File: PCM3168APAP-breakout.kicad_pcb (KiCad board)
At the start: 4 copper layers, 133.6 x 66.2 mm, 206 parts, among them IC101 PCM3168APAP, IC102 SN74LVC2G34DRLR, J1 ~{RESET}, J101 I^{2}S, J102 I^{2}C, J103 DIN, J104 DOUT, J201 ANALOG_IN1, J202 ANALOG_IN2, J203 ANALOG_IN3, J301 OUTPUT1-4, J302 OUTPUT5-8, J401 POWER IN, U201 OPA4134UA, U202 OPA2134, U301 OPA4134UA, U302 OPA4134UA, U401 AMS1117-5.0, U402 AMS1117-3.3

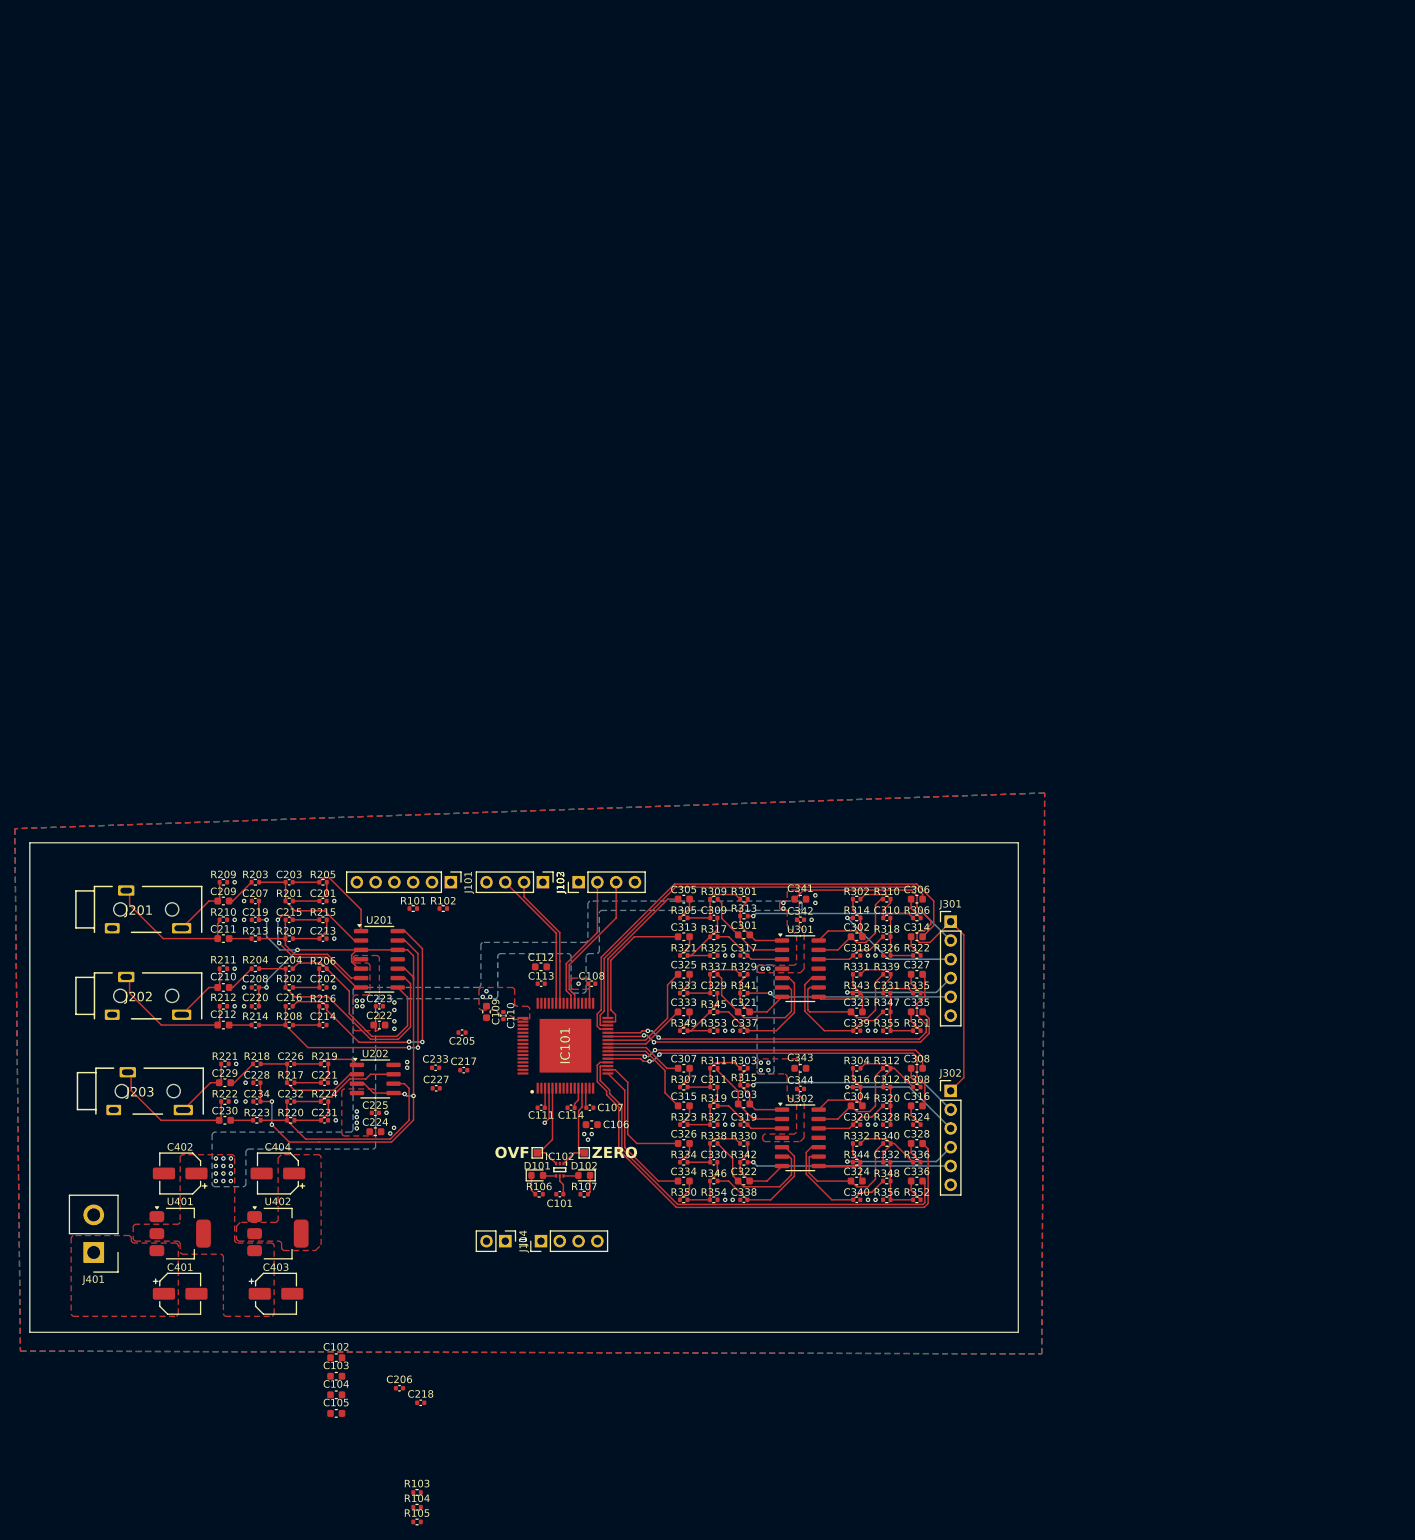
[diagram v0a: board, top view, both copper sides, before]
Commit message: finished routin, updated schematic, added PDF
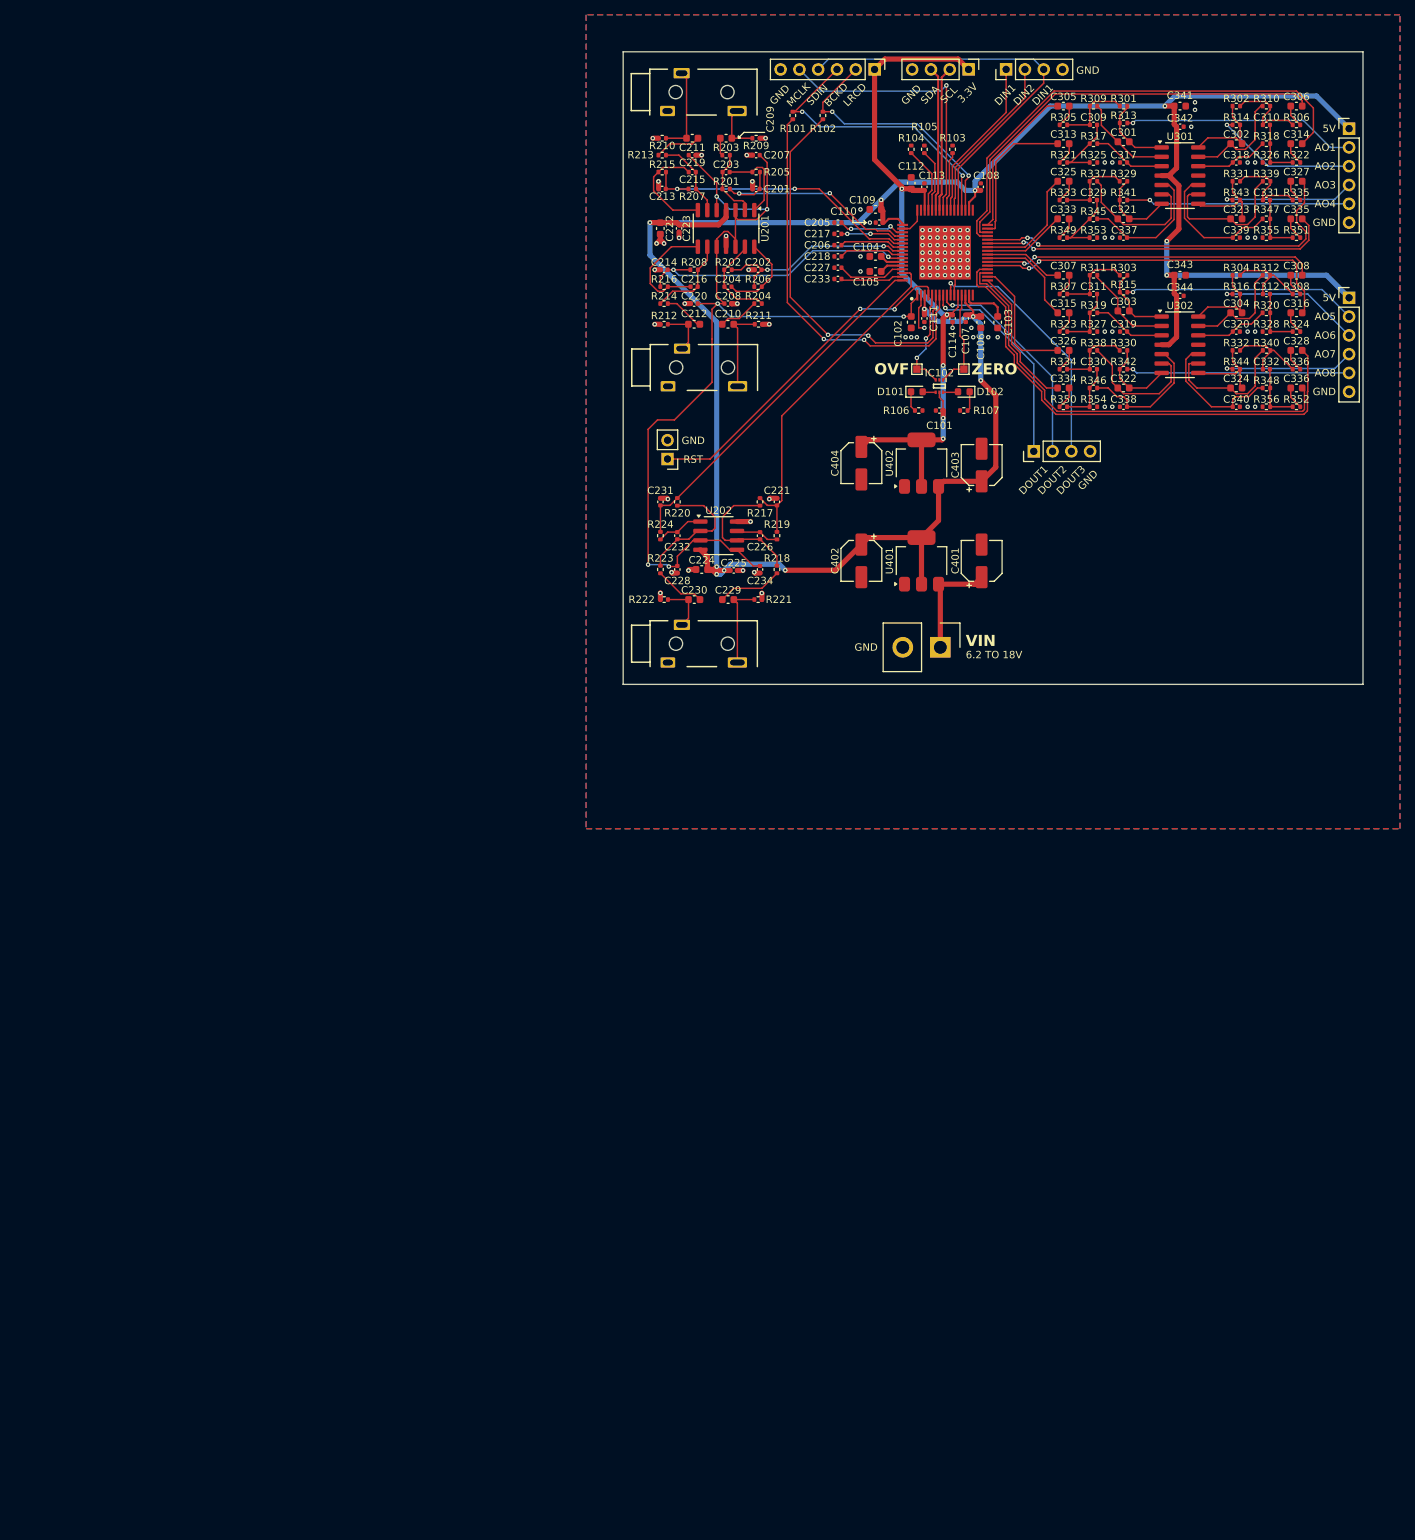
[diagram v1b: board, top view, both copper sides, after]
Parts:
- moved R105 197.8 mm to (140.7, 43.2), turned to -90 degrees
- moved R103 195.4 mm to (144.5, 43.2), turned to -90 degrees
- moved R104 195.3 mm to (138.9, 43.2), turned to -90 degrees
- moved C105 170.7 mm to (134.1, 59.7), turned to 180 degrees
- moved C104 170.3 mm to (134.1, 57.7), turned to 180 degrees
- moved C103 168.2 mm to (150.6, 66.5), turned to -90 degrees
- moved C206 165.5 mm to (129.0, 56.1), turned to 180 degrees
- moved C218 164.9 mm to (129.0, 57.7), turned to 180 degrees
- moved C102 160.1 mm to (138.9, 66.5), turned to -90 degrees
- moved C403 147.1 mm to (148.5, 85.9), turned to 90 degrees
- moved C401 146.8 mm to (148.5, 98.8), turned to 90 degrees
- moved J401 140.7 mm to (142.9, 110.5), turned to -90 degrees
- moved U402 135.7 mm to (140.3, 85.6), turned to 90 degrees
- moved U401 135.3 mm to (140.3, 98.8), turned to 90 degrees
- moved J201 133.6 mm to (106.0, 38.0)
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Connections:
- C204 pad 1: Net-(U201C--) -> Net-(U201D--)
- C216 pad 1: Net-(U201D--) -> Net-(U201C--)
- C226 pad 1: Net-(U202A--) -> Net-(U202B--)
- C232 pad 1: Net-(U202B--) -> Net-(U202A--)
- R202 pad 1: Net-(U201C--) -> Net-(U201D--)
- R204 pad 2: Net-(U201C--) -> Net-(U201D--)
- R208 pad 1: Net-(U201D--) -> Net-(U201C--)
- R214 pad 2: Net-(U201D--) -> Net-(U201C--)
- R217 pad 1: Net-(U202A--) -> Net-(U202B--)
- R218 pad 2: Net-(U202A--) -> Net-(U202B--)
- R220 pad 1: Net-(U202B--) -> Net-(U202A--)
- R223 pad 2: Net-(U202B--) -> Net-(U202A--)
- U201 pad 14: Net-(C216-Pad2) -> Net-(C204-Pad2)
- U201 pad 8: Net-(C204-Pad2) -> Net-(C216-Pad2)
- U202 pad 1: Net-(C226-Pad2) -> Net-(C232-Pad2)
- U202 pad 7: Net-(C232-Pad2) -> Net-(C226-Pad2)
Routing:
- net +5V: track 63.5 -> 344.2 mm, vias 35 -> 13
- net +3.3V: track 5.52 -> 99.4 mm, vias 0 -> 5
- net /SDIN: track 0.00 -> 55.5 mm
- net /BCK_ADC: track 0.00 -> 54.1 mm, vias 0 -> 2
- net /LRCK_ADC: track 0.00 -> 53.9 mm, vias 0 -> 2
- net /Analog Inputs/VIN6+: track 6.53 -> 48.9 mm
- net /~{RST}: track 4.93 -> 46.2 mm, vias 1 -> 2
- net /Analog Inputs/VIN5+: track 6.53 -> 46.3 mm
- net /BCK_DAC: track 0.00 -> 39.6 mm, vias 0 -> 2
- net /Analog Inputs/VCOMAD: track 103.4 -> 141.9 mm, vias 7 -> 6
- net /MCLK: track 0.00 -> 38.4 mm, vias 0 -> 1
- net GND: track 0.00 -> 36.4 mm, vias 45 -> 106
- net /LRCK_DAC: track 0.00 -> 35.7 mm, vias 0 -> 2
- net /DOUT3: track 0.00 -> 34.5 mm, vias 0 -> 1
- net /Analog Inputs/VIN4+: track 6.13 -> 38.8 mm, vias 0 -> 2
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- removed copper zone on F.Cu, net +3.3V
- removed copper zone on B.Cu, net +5V
- removed copper zone on F.Cu, net +5V
- removed copper zone on F.Cu, net /Power/V_EXT
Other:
- board size 133.6 x 66.2 mm -> 100 x 85.5 mm
- board text added: "3.3V"
- board text added: "5V"
- board text added: "6.2 TO 18V"
- board text added: "AO1"
- board text added: "AO2"
- board text added: "AO3"
- board text added: "AO4"
- board text added: "AO5"
- board text added: "AO6"
- board text added: "AO7"
- board text added: "AO8"
- board text added: "BCKD"
- board text added: "DIN1"
- board text added: "DIN2"
- board text added: "DOUT1"
- board text added: "DOUT2"
- board text added: "DOUT3"
- board text added: "GND"
- board text added: "LRCD"
- board text added: "MCLK"
- board text added: "RST"
- board text added: "SCL"
- board text added: "SDA"
- board text added: "SDIN"
- board text added: "VIN"
